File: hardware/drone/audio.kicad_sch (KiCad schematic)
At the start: 20 parts, among them U11 TAC5111, U12 LM4670SD/NOPB

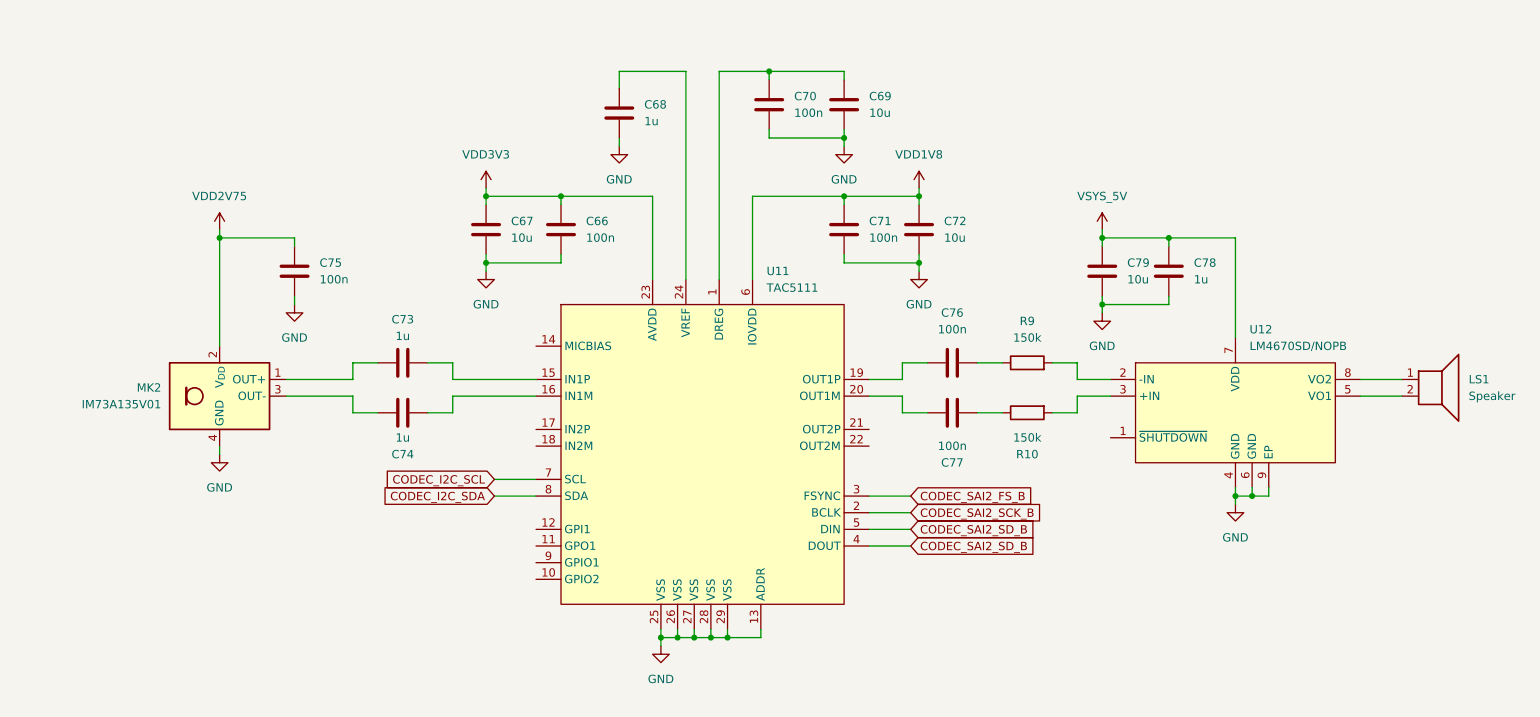
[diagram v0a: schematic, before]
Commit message: Finished GNSS, did more pinmuxxing
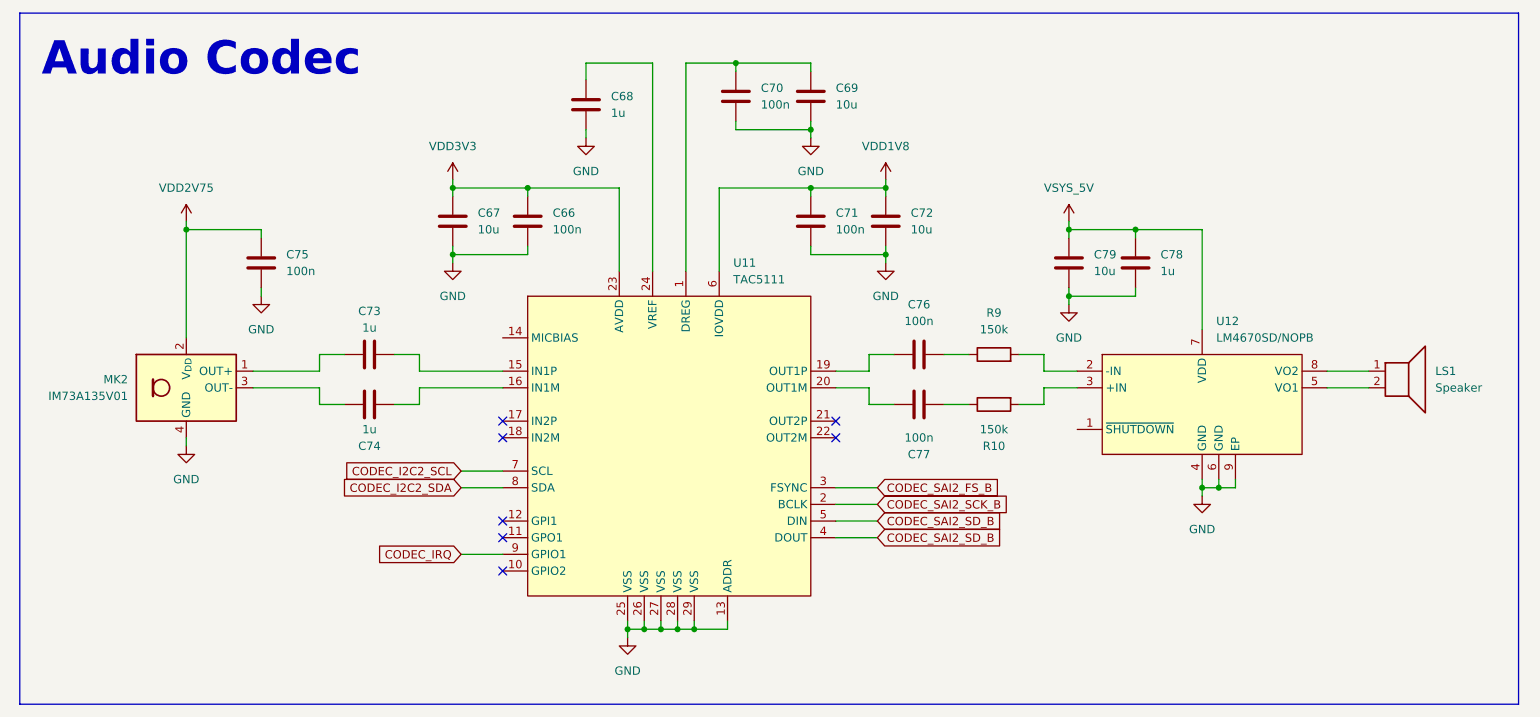
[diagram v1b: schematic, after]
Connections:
- net CODEC_IRQ: now reaches U11.9 (GPIO1)
- net CODEC_I2C_SCL renamed CODEC_I2C2_SCL
- net CODEC_I2C_SDA renamed CODEC_I2C2_SDA
- no-connect marks 0 -> 7
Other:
- note added: "Audio Codec"
- moved on the sheet: C66, C67, C68, C69, C70, C71, C72, C73, C74, C75, C76, C77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
